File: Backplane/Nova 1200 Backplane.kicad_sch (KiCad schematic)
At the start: 46 parts, among them J1 Conn_02x40_Odd_Even, J10 Conn_01x10, J11 Conn_01x10, J12 Conn_01x10, J13 Conn_01x10, J14 Conn_01x10, J15 Conn_01x10, J16 Conn_01x10, J17 Conn_01x10, J18 Conn_01x10, J19 Conn_01x10, J1A1 Conn_01x40, J1A2 Conn_01x40, J1A3 Conn_01x40, J1A4 Conn_01x40, J1A5 Conn_01x40, J1B1 Conn_01x40, J1B2 Conn_01x40, J1B3 Conn_01x40, J1B4 Conn_01x40, J1B5 Conn_01x40, J2 DG Nova Card-Edge 81-100, J20 Conn_01x10, J21 Conn_01x10, J22 Conn_01x10, J23 Conn_01x10, J24 Conn_01x10, J2A1 Conn_01x40, J2A2 Conn_01x40, J2A3 Conn_01x40, J2A4 Conn_01x40, J2A5 Conn_01x40, J2B1 Conn_01x40, J2B2 Conn_01x40, J2B3 Conn_01x40, J2B4 Conn_01x40, J2B5 Conn_01x40, J3 Conn_02x40_Odd_Even, J4 DG Nova Card-Edge 81-100, J5 Conn_01x10, J6 Conn_01x10, J7 Conn_01x10, J8 Conn_01x10, J9 Conn_01x10

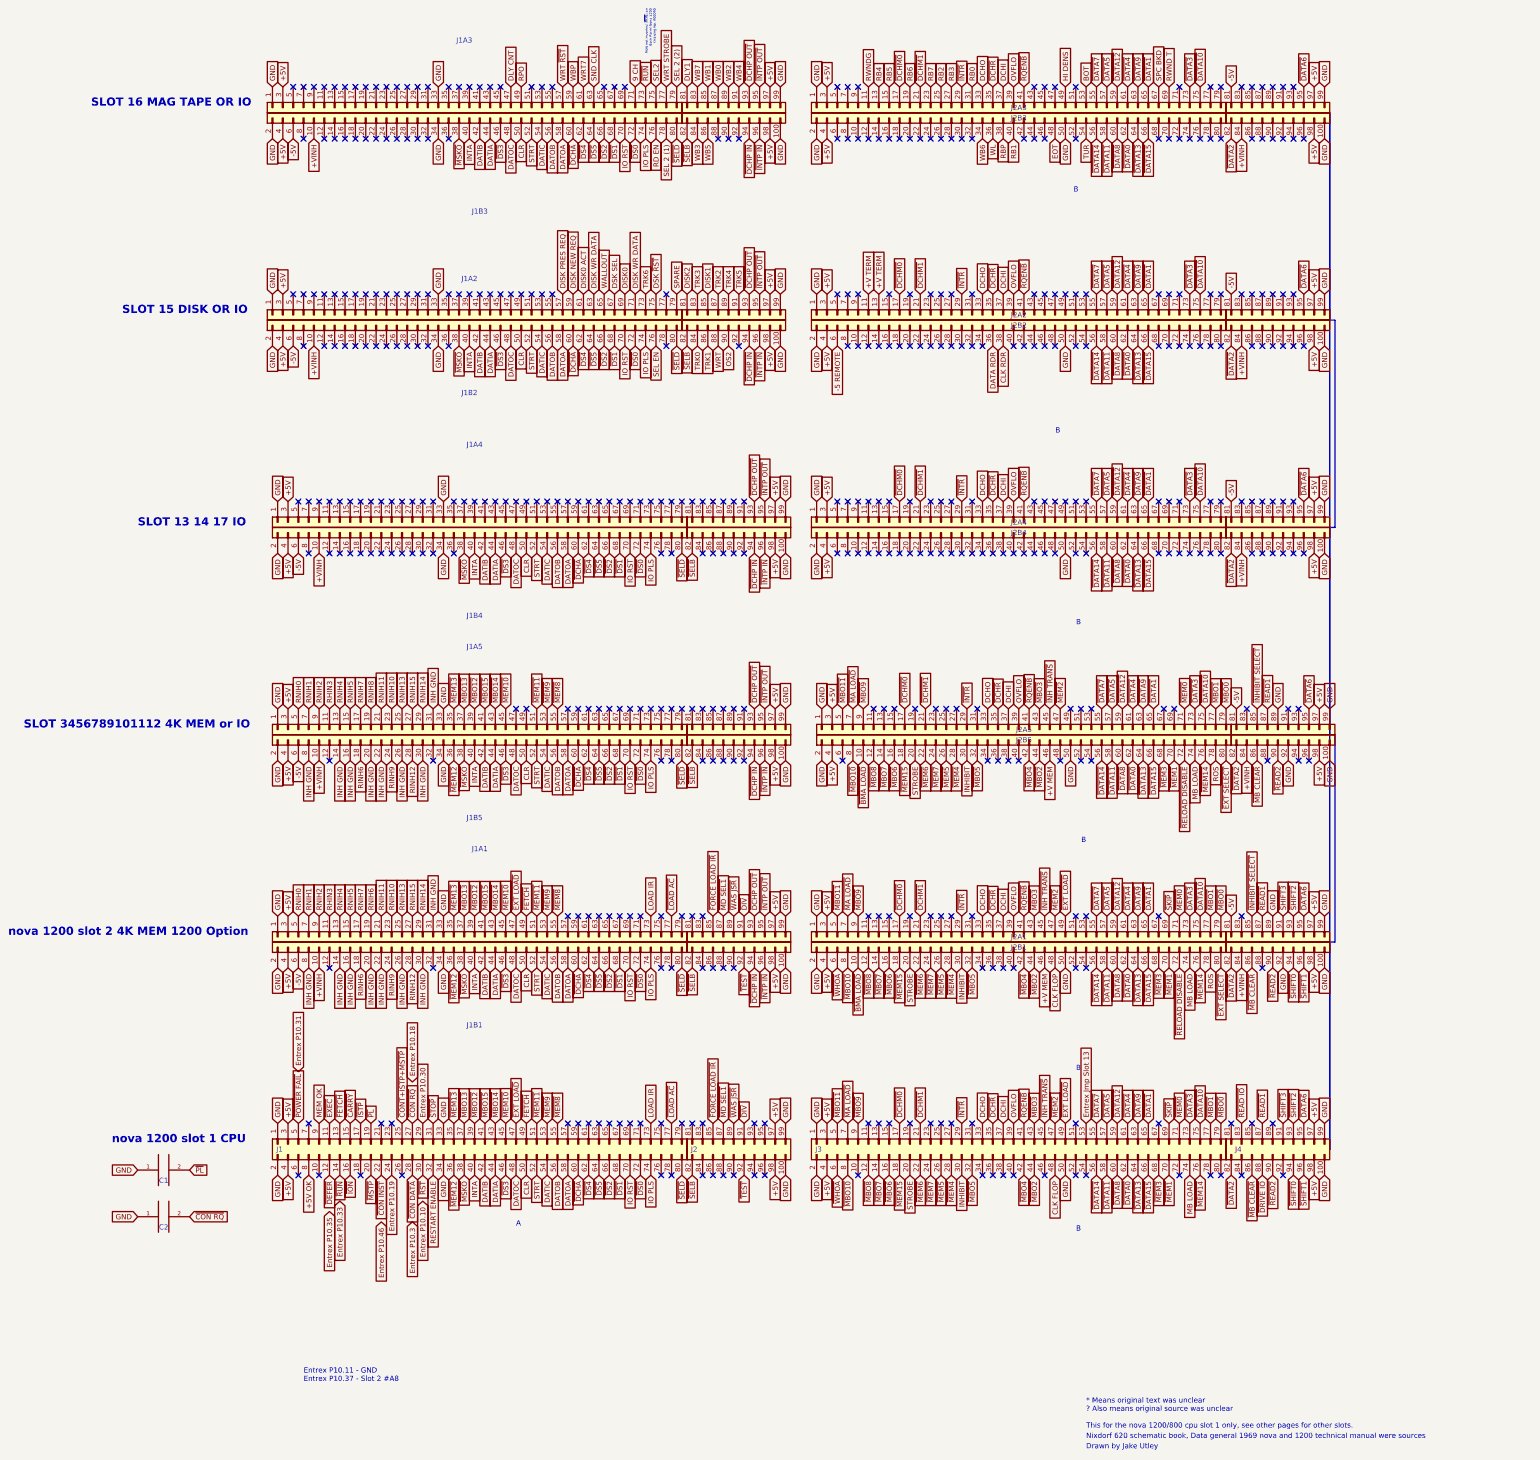
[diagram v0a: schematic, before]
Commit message: yo
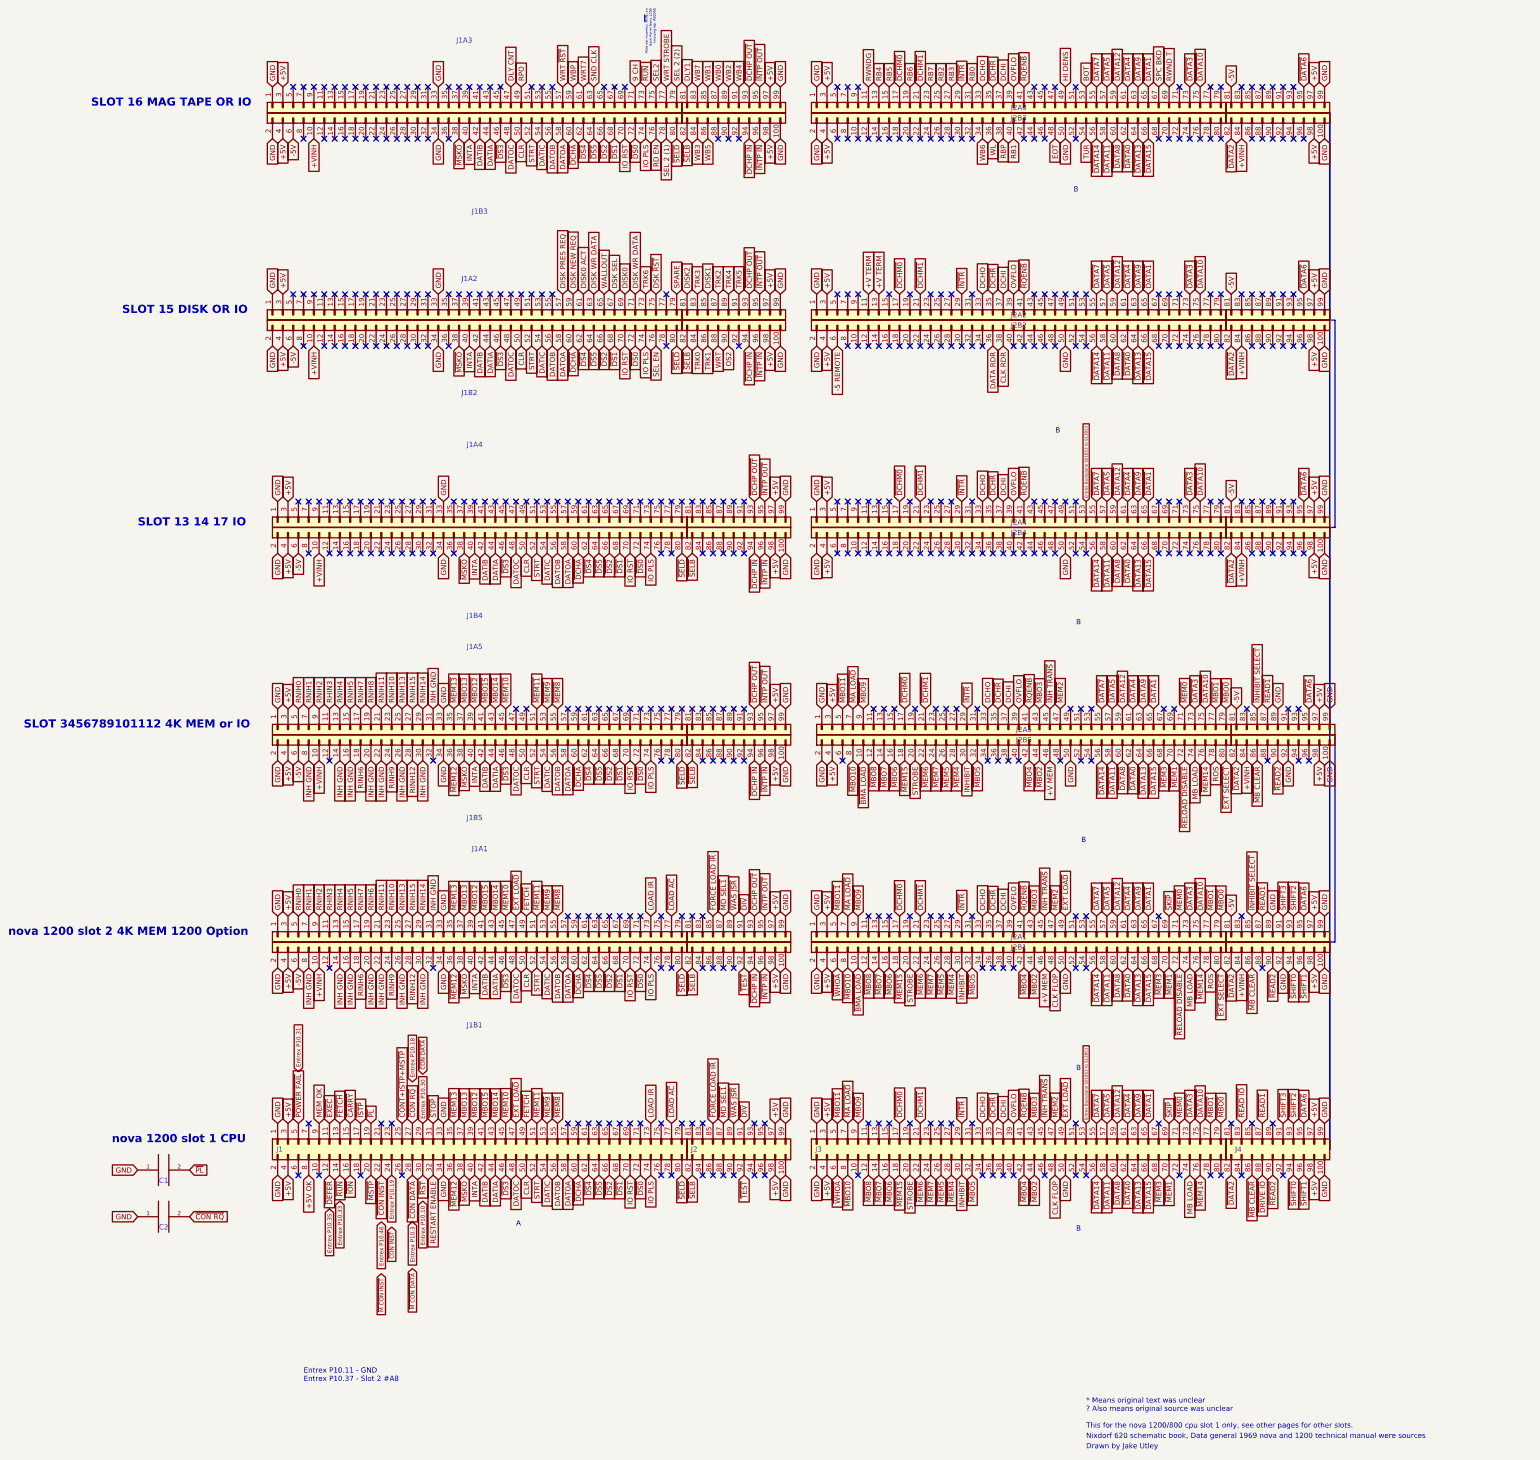
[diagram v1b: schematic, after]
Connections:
- net Entrex Jmp Slot 13 is gone; now on net Entrex Backplane S01B53 to S13B53: J3.53 (Pin_53)
- net Entrex Backplane S01B53 to S13B53: now reaches J2A4.53 (Pin_27)
- no-connect marks 468 -> 467
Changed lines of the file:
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@@
   (no_connect (at 327.66 289.56))
   (no_connect (at 246.38 99.06))
-  (no_connect (at 281.94 137.16))
   (no_connect (at 95.25 35.56))
   (no_connect (at 116.84 137.16))
@@
   )
   (global_label "Entrex P10.18" (shape input) (at 116.84 279.4 90) (fields_autoplaced)
-    (effects (font (size 1.27 1.27)) (justify left))
-    (property "Intersheetrefs" "${INTERSHEET_REFS}" (at 116.84 263.0928 90)
+    (effects (font (size 1 1)) (justify left))
+    (property "Intersheetrefs" "${INTERSHEET_REFS}" (at 116.84 266.5597 90)
       (effects (font (size 1.27 1.27)) (justify left) hide)
     )
@@
     )
   )
+  (global_label "Entrex Backplane S01B53 to S13B53" (shape input) (at 281.94 289.56 90) (fields_autoplaced)
+    (effects (font (size 0.7 0.7)) (justify left))
+    (property "Intersheetrefs" "${INTERSHEET_REFS}" (at 281.94 268.545 90)
+      (effects (font (size 1.27 1.27)) (justify left) hide)
+    )
+  )
   (global_label "~{DS3}" (shape input) (at 139.7 302.26 270) (fields_autoplaced)
     (effects (font (size 1.27 1.27)) (justify right))
@@
   )
   (global_label "Entrex P10.31" (shape input) (at 88.9 276.86 90) (fields_autoplaced)
-    (effects (font (size 1.27 1.27)) (justify left))
-    (property "Intersheetrefs" "${INTERSHEET_REFS}" (at 88.9 260.5528 90)
+    (effects (font (size 1 1)) (justify left))
+    (property "Intersheetrefs" "${INTERSHEET_REFS}" (at 88.9 264.0197 90)
       (effects (font (size 1.27 1.27)) (justify left) hide)
     )
@@
     )
   )
+  (global_label "~{M CON DATA}" (shape input) (at 116.84 325.12 270) (fields_autoplaced)
+    (effects (font (size 1 1)) (justify right))
+    (property "Intersheetrefs" "${INTERSHEET_REFS}" (at 116.84 336.3221 90)
+      (effects (font (size 1.27 1.27)) (justify right) hide)
+    )
+  )
   (global_label "~{DCHA}" (shape input) (at 157.48 200.66 270) (fields_autoplaced)
     (effects (font (size 1.27 1.27)) (justify right))
@@
   )
   (global_label "Entrex P10.10" (shape input) (at 119.38 308.61 270) (fields_autoplaced)
-    (effects (font (size 1.27 1.27)) (justify right))
-    (property "Intersheetrefs" "${INTERSHEET_REFS}" (at 119.38 324.9172 90)
+    (effects (font (size 1 1)) (justify right))
+    (property "Intersheetrefs" "${INTERSHEET_REFS}" (at 119.38 321.4503 90)
       (effects (font (size 1.27 1.27)) (justify right) hide)
     )
@@
   )
   (global_label "Entrex P10.33" (shape input) (at 99.06 308.61 270) (fields_autoplaced)
-    (effects (font (size 1.27 1.27)) (justify right))
-    (property "Intersheetrefs" "${INTERSHEET_REFS}" (at 99.06 324.9172 90)
+    (effects (font (size 1 1)) (justify right))
+    (property "Intersheetrefs" "${INTERSHEET_REFS}" (at 99.06 321.4503 90)
       (effects (font (size 1.27 1.27)) (justify right) hide)
     )
@@
     )
   )
+  (global_label "~{M CON INST}" (shape input) (at 109.22 326.39 270) (fields_autoplaced)
+    (effects (font (size 1 1)) (justify right))
+    (property "Intersheetrefs" "${INTERSHEET_REFS}" (at 109.22 337.3541 90)
+      (effects (font (size 1.27 1.27)) (justify right) hide)
+    )
+  )
   (global_label "~{DATA8}" (shape input) (at 289.56 48.26 270) (fields_autoplaced)
     (effects (font (size 1.27 1.27)) (justify right))
@@
   )
   (global_label "Entrex P10.3" (shape input) (at 116.84 313.69 270) (fields_autoplaced)
-    (effects (font (size 1.27 1.27)) (justify right))
-    (property "Intersheetrefs" "${INTERSHEET_REFS}" (at 116.84 328.7877 90)
+    (effects (font (size 1 1)) (justify right))
+    (property "Intersheetrefs" "${INTERSHEET_REFS}" (at 116.84 325.5779 90)
       (effects (font (size 1.27 1.27)) (justify right) hide)
     )
@@
     )
   )
-  (global_label "Entrex P10.35" (shape input) (at 96.52 311.15 270) (fields_autoplaced)
-    (effects (font (size 1.27 1.27)) (justify right))
-    (property "Intersheetrefs" "${INTERSHEET_REFS}" (at 96.52 327.4572 90)
+  (global_label "Entrex P10.35" (shape input) (at 96.52 310.515 270) (fields_autoplaced)
+    (effects (font (size 1 1)) (justify right))
+    (property "Intersheetrefs" "${INTERSHEET_REFS}" (at 96.52 323.3553 90)
       (effects (font (size 1.27 1.27)) (justify right) hide)
     )
@@
     )
   )
+  (global_label "~{CON INST}" (shape input) (at 111.76 314.96 270) (fields_autoplaced)
+    (effects (font (size 1 1)) (justify right))
+    (property "Intersheetrefs" "${INTERSHEET_REFS}" (at 111.76 324.1812 90)
+      (effects (font (size 1.27 1.27)) (justify right) hide)
+    )
+  )
   (global_label "~{DATA7}" (shape input) (at 284.48 86.36 90) (fields_autoplaced)
     (effects (font (size 1.27 1.27)) (justify left))
@@
     )
   )
+  (global_label "Entrex Backplane S01B53 to S13B53" (shape input) (at 281.94 137.16 90) (fields_autoplaced)
+    (effects (font (size 0.7 0.7)) (justify left))
+    (property "Intersheetrefs" "${INTERSHEET_REFS}" (at 281.94 116.145 90)
+      (effects (font (size 1.27 1.27)) (justify left) hide)
+    )
+  )
   (global_label "INH GND" (shape input) (at 101.6 251.46 270) (fields_autoplaced)
     (effects (font (size 1.27 1.27)) (justify right))
@@
   )
   (global_label "Entrex P10.19" (shape input) (at 111.76 302.26 270) (fields_autoplaced)
-    (effects (font (size 1.27 1.27)) (justify right))
-    (property "Intersheetrefs" "${INTERSHEET_REFS}" (at 111.76 318.5672 90)
+    (effects (font (size 1 1)) (justify right))
+    (property "Intersheetrefs" "${INTERSHEET_REFS}" (at 111.76 315.1003 90)
       (effects (font (size 1.27 1.27)) (justify right) hide)
     )
@@
   )
   (global_label "Entrex P10.46" (shape input) (at 109.22 313.69 270) (fields_autoplaced)
-    (effects (font (size 1.27 1.27)) (justify right))
-    (property "Intersheetrefs" "${INTERSHEET_REFS}" (at 109.22 329.9972 90)
+    (effects (font (size 1 1)) (justify right))
+    (property "Intersheetrefs" "${INTERSHEET_REFS}" (at 109.22 326.5303 90)
       (effects (font (size 1.27 1.27)) (justify right) hide)
     )
@@
     )
   )
-  (global_label "Entrex Jmp Slot 13" (shape input) (at 281.94 289.56 90) (fields_autoplaced)
-    (effects (font (size 1.27 1.27)) (justify left))
-    (property "Intersheetrefs" "${INTERSHEET_REFS}" (at 281.94 268.4633 90)
+  (global_label "~{CON DATA}" (shape input) (at 119.38 277.495 90) (fields_autoplaced)
+    (effects (font (size 1 1)) (justify left))
+    (property "Intersheetrefs" "${INTERSHEET_REFS}" (at 119.38 268.0358 90)
       (effects (font (size 1.27 1.27)) (justify left) hide)
     )
@@
   )
   (global_label "Entrex P10.30" (shape input) (at 119.38 289.56 90) (fields_autoplaced)
-    (effects (font (size 1.27 1.27)) (justify left))
-    (property "Intersheetrefs" "${INTERSHEET_REFS}" (at 119.38 273.2528 90)
+    (effects (font (size 1 1)) (justify left))
+    (property "Intersheetrefs" "${INTERSHEET_REFS}" (at 119.38 276.7197 90)
       (effects (font (size 1.27 1.27)) (justify left) hide)
     )
